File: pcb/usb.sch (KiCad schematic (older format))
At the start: 7 parts, among them P1 USB

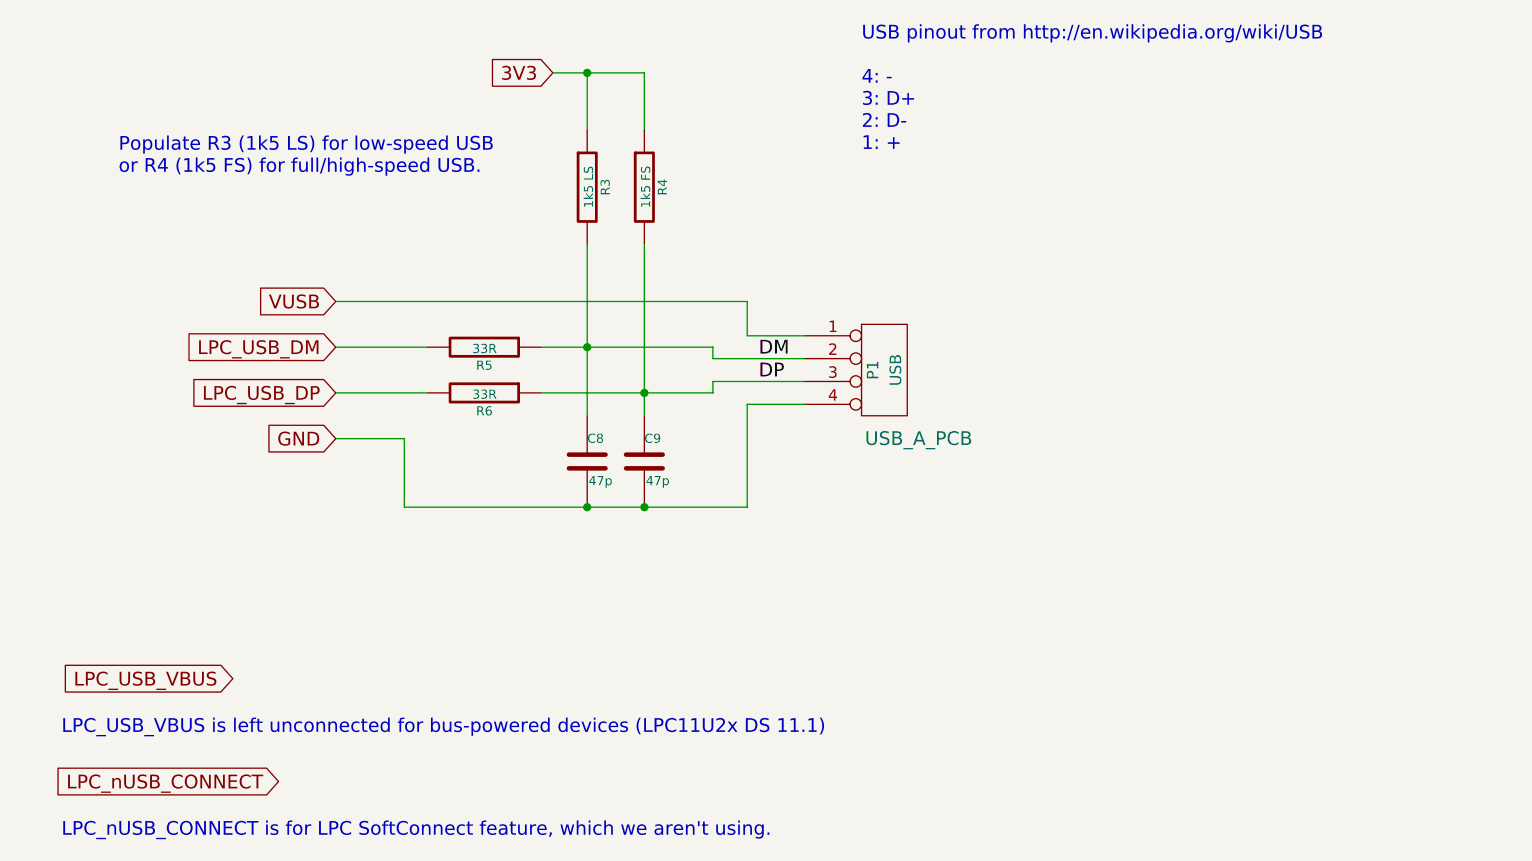
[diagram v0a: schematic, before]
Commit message: pcb work from last night
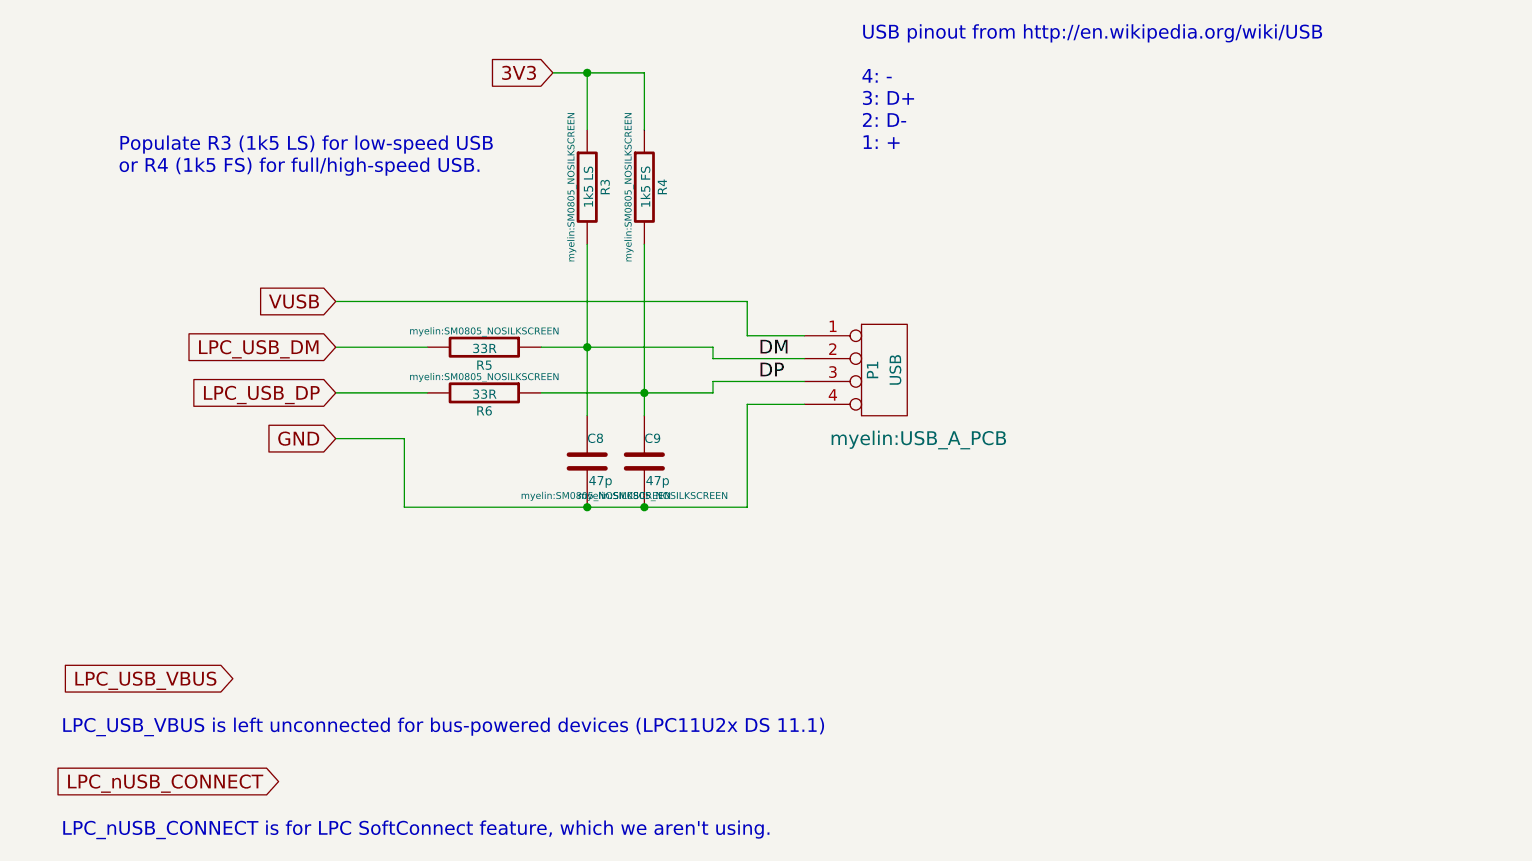
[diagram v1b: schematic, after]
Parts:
- C8, C9, R3, R4, R5, R6: footprint ~ -> myelin:SM0805_NOSILKSCREEN
- P1: footprint USB_A_PCB -> myelin:USB_A_PCB
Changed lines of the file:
@@
 F 0 "P1" V 6100 3100 50  0000 C CNN
 F 1 "USB" V 6200 3100 50  0000 C CNN
-F 2 "USB_A_PCB" H 6300 2800 60  0000 C CNN
+F 2 "myelin:USB_A_PCB" H 6300 2800 60  0000 C CNN
 F 3 "" H 6150 3100 60  0000 C CNN
 	1    6150 3100
@@
 F 0 "R5" V 4480 3000 40  0000 C CNN
 F 1 "33R" V 4407 3001 40  0000 C CNN
-F 2 "~" V 4330 3000 30  0000 C CNN
+F 2 "myelin:SM0805_NOSILKSCREEN" V 4330 3000 30  0000 C CNN
 F 3 "~" H 4400 3000 30  0000 C CNN
 	1    4400 3000
@@
 F 0 "R6" V 4480 3200 40  0000 C CNN
 F 1 "33R" V 4407 3201 40  0000 C CNN
-F 2 "~" V 4330 3200 30  0000 C CNN
+F 2 "myelin:SM0805_NOSILKSCREEN" V 4330 3200 30  0000 C CNN
 F 3 "~" H 4400 3200 30  0000 C CNN
 	1    4400 3200
@@
 F 0 "R3" V 4930 2300 40  0000 C CNN
 F 1 "1k5 LS" V 4857 2301 40  0000 C CNN
-F 2 "~" V 4780 2300 30  0000 C CNN
+F 2 "myelin:SM0805_NOSILKSCREEN" V 4780 2300 30  0000 C CNN
 F 3 "~" H 4850 2300 30  0000 C CNN
 	1    4850 2300
@@
 F 0 "R4" V 5180 2300 40  0000 C CNN
 F 1 "1k5 FS" V 5107 2301 40  0000 C CNN
-F 2 "~" V 5030 2300 30  0000 C CNN
+F 2 "myelin:SM0805_NOSILKSCREEN" V 5030 2300 30  0000 C CNN
 F 3 "~" H 5100 2300 30  0000 C CNN
 	1    5100 2300
@@
 F 0 "C9" H 5100 3600 40  0000 L CNN
 F 1 "47p" H 5106 3415 40  0000 L CNN
-F 2 "~" H 5138 3350 30  0000 C CNN
+F 2 "myelin:SM0805_NOSILKSCREEN" H 5138 3350 30  0000 C CNN
 F 3 "~" H 5100 3500 60  0000 C CNN
 	1    5100 3500
@@
 F 0 "C8" H 4850 3600 40  0000 L CNN
 F 1 "47p" H 4856 3415 40  0000 L CNN
-F 2 "~" H 4888 3350 30  0000 C CNN
+F 2 "myelin:SM0805_NOSILKSCREEN" H 4888 3350 30  0000 C CNN
 F 3 "~" H 4850 3500 60  0000 C CNN
 	1    4850 3500
